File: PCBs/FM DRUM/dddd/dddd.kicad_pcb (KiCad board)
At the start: 2 copper layers, 66 x 43.2 mm, 44 parts, among them J1 Conn_02x12_Odd_Even, J2 Conn_01x03, J3 Conn_01x03, J4 Conn_01x03, J5 Conn_01x03, J6 Conn_01x03, J7 Conn_01x03, SW1 SW_DIP_x06, U1 LM555xM, U2 LM555xM, U3 MCP46x2, U4 LM555xM, U5 LM555xM, U6 MCP46x2, U7 MCP46x2, U8 TL072

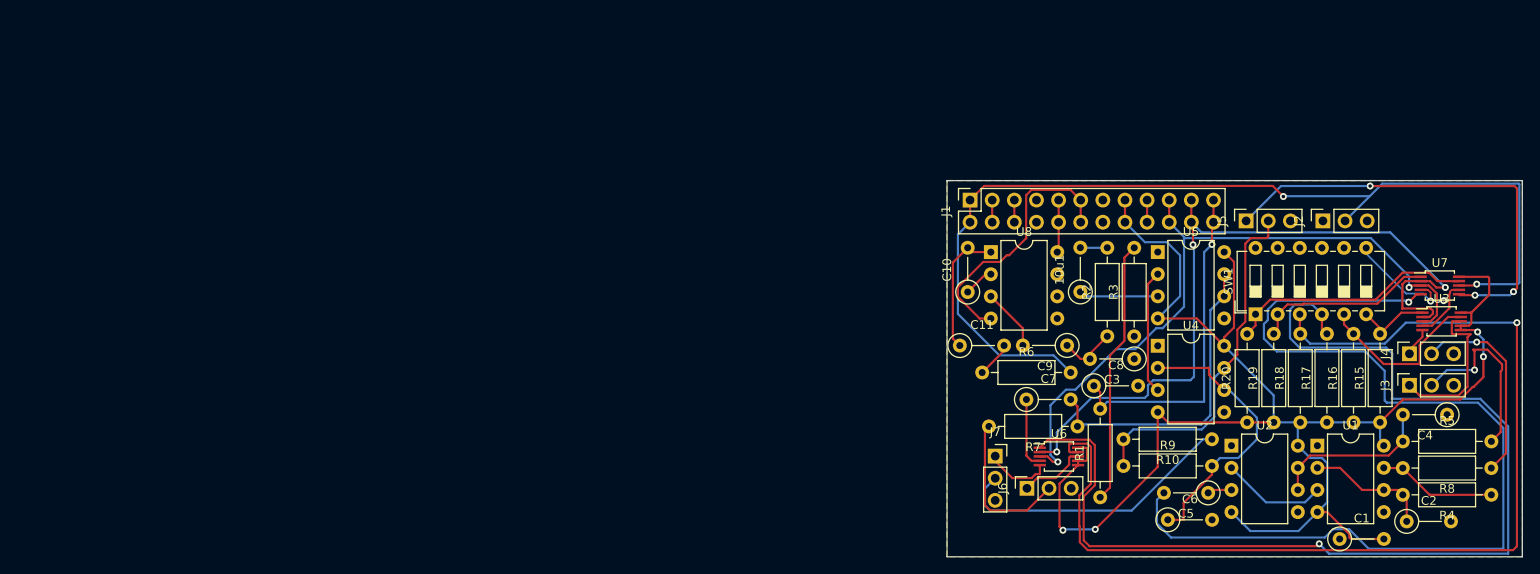
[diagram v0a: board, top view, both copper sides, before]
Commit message: Add files via upload
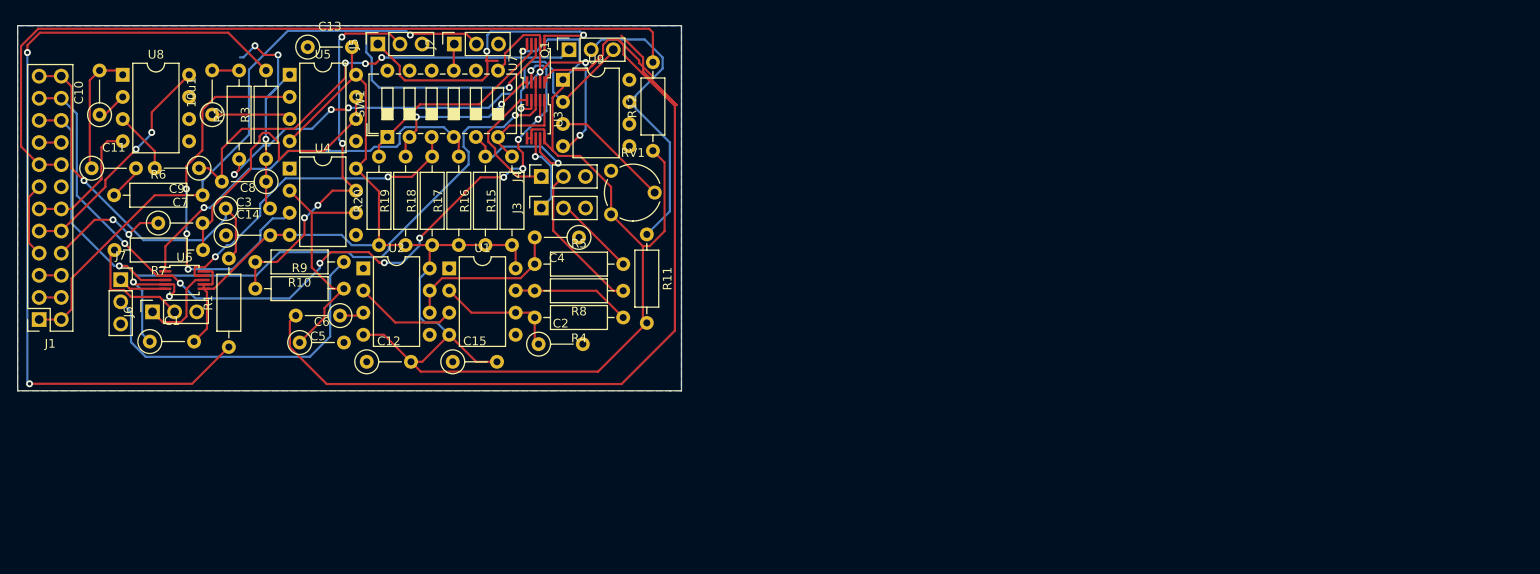
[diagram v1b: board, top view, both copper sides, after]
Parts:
- added C12: 22p, Resistor_THT:R_Axial_DIN0207_L6.3mm_D2.5mm_P5.08mm_Vertical, F.Cu at (172.2, 71.6)
- added C13: 22p, Resistor_THT:R_Axial_DIN0207_L6.3mm_D2.5mm_P5.08mm_Vertical, F.Cu at (165.4, 35.5)
- added C14: 22p, Resistor_THT:R_Axial_DIN0207_L6.3mm_D2.5mm_P5.08mm_Vertical, F.Cu at (156.0, 57.1)
- added C15: 22p, Resistor_THT:R_Axial_DIN0207_L6.3mm_D2.5mm_P5.08mm_Vertical, F.Cu at (182.0, 71.6)
- added Q1: 2N3904, Connector_PinSocket_2.54mm:PinSocket_1x03_P2.54mm_Vertical, F.Cu at (195.4, 35.8)
- added R11: 10k, Resistor_THT:R_Axial_DIN0207_L6.3mm_D2.5mm_P10.16mm_Horizontal, F.Cu at (204.3, 57.0)
- added R12: 47, Resistor_THT:R_Axial_DIN0207_L6.3mm_D2.5mm_P10.16mm_Horizontal, F.Cu at (205.0, 47.4)
- added RV1: R_POT, Potentiometer_THT:Potentiometer_Piher_PT-6-V_Vertical, F.Cu at (200.2, 54.7)
- added U9: AD8561, Package_DIP:DIP-8_W7.62mm, F.Cu at (194.7, 39.2)
- moved C1 138.4 mm to (147.2, 69.3)
- moved J1 107.7 mm to (134.6, 66.8), turned to 180 degrees
- moved U7 106.9 mm to (191.6, 37.3), turned to 90 degrees
- moved U3 106.5 mm to (191.6, 43.8), turned to 270 degrees
- moved J6 102.4 mm to (147.6, 65.9)
- moved J7 102.4 mm to (143.9, 62.2)
- moved R7 102.4 mm to (153.4, 58.8)
- moved U6 102.4 mm to (151.2, 62.2)
- moved J2 101.8 mm to (182.2, 35.1)
- moved J5 101.7 mm to (173.4, 35.1)
- moved C6 101.7 mm to (164.5, 69.4)
- moved 10u1 101.7 mm to (154.4, 43.2)
- moved C10 101.7 mm to (141.5, 43.2)
- moved C11 101.7 mm to (140.6, 49.4)
- moved C2 101.7 mm to (191.9, 69.6)
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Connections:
- C1 pad 2: 5V -> 5V_CL
- R15 pad 1: 5V -> 5V_CL
- R16 pad 1: 5V -> 5V_CL
- R17 pad 1: 5V -> 5V_CL
- R18 pad 1: 5V -> 5V_CL
- R19 pad 1: 5V -> 5V_CL
- R2 pad 1: LPG_OUT -> VACTROL_OUT
- R20 pad 1: 5V -> 5V_CL
- U1 pad 4: 5V -> 5V_CL
- U1 pad 8: 5V -> 5V_CL
- U2 pad 4: 5V -> 5V_CL
- U2 pad 8: 5V -> 5V_CL
- U3 pad 10: 5V -> 5V_CL
- U3 pad 6: 5V -> 5V_CL
- U3 pad 7: 5V -> 5V_CL
- U4 pad 4: 5V -> 5V_CL
- U4 pad 8: 5V -> 5V_CL
- U5 pad 4: 5V -> 5V_CL
- U5 pad 8: 5V -> 5V_CL
- U6 pad 10: 5V -> 5V_CL
- U6 pad 6: 5V -> 5V_CL
- U6 pad 7: 5V -> 5V_CL
- U7 pad 10: 5V -> 5V_CL
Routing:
- net 5V_CL: track 0.00 -> 216.6 mm, vias 0 -> 1
- net 5V: track 182.3 -> 94.0 mm, vias 4 -> 0
- net A3: track 121.2 -> 37.5 mm, vias 1 -> 2
- net A2: track 125.1 -> 45.4 mm
- net GND: track 30.0 -> 104.8 mm, vias 2 -> 11
- net Net-(R1-Pad1): track 30.3 -> 93.4 mm, vias 0 -> 2
- net VACTROL_OUT: track 0.00 -> 57.8 mm, vias 0 -> 3
- net LPG_OUT: track 7.30 -> 52.7 mm, vias 0 -> 3
- net Net-(Q1-Pad2): track 0.00 -> 34.5 mm
- net Net-(U4-Pad3): track 14.2 -> 44.8 mm, vias 0 -> 3
- net +12V: track 6.04 -> 26.5 mm, vias 0 -> 2
- net A_OUT_L: track 116.6 -> 100.4 mm
- net -12V: track 30.5 -> 15.0 mm
- net Net-(RV1-Pad2): track 0.00 -> 13.8 mm
- net APC2_IN: track 51.4 -> 38.1 mm, vias 3 -> 2
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- added copper zone on B.Cu, net GND
- removed copper zone on F.Cu, net GND
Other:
- board size 66 x 43.2 mm -> 76.2 x 41.9 mm
